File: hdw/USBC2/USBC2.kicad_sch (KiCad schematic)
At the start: 7 parts, among them J1 Conn_01x02, J2 Conn_01x02, J3 Conn_01x02, J4 Conn_01x02, P1 USB_C_2.0

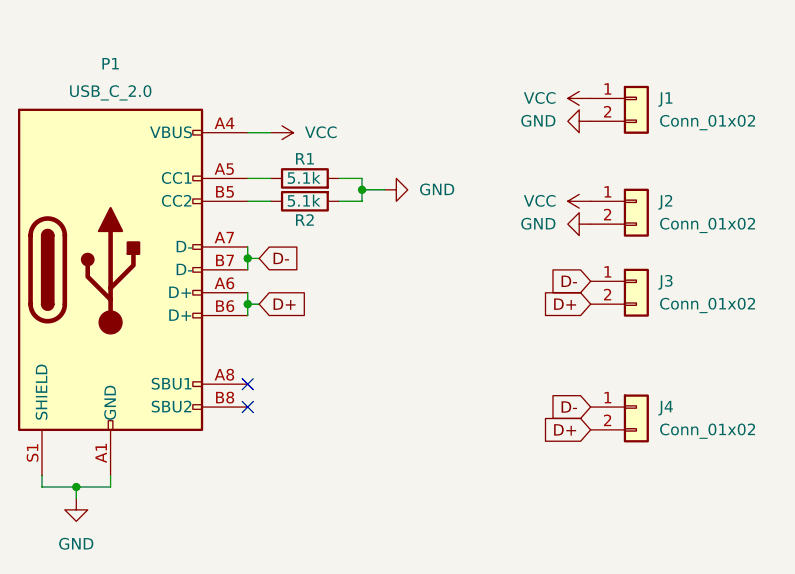
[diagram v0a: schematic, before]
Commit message: Save changes at: 1748195240
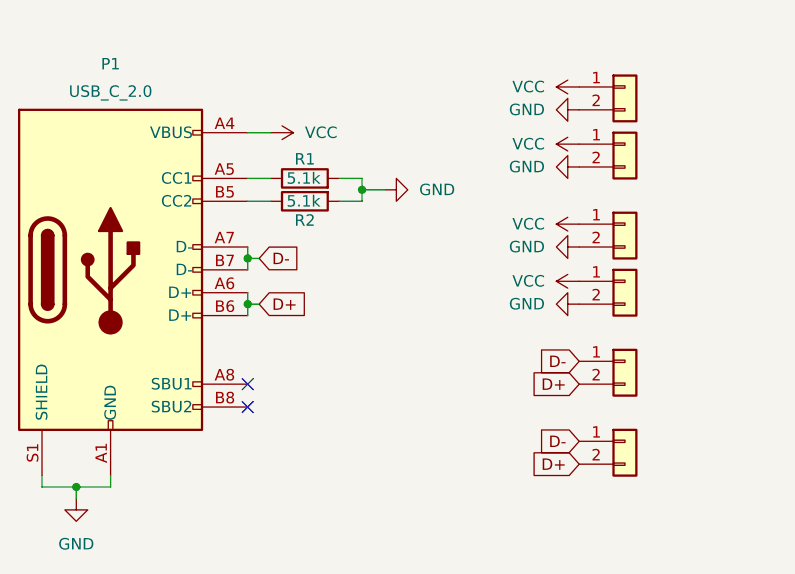
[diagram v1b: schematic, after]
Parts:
- added J5, J6: Conn_01x02, Connector_PinHeader_2.54mm:PinHeader_1x02_P2.54mm_Vertical, symbol Connector_Generic:Conn_01x02
- P1: footprint Connector_USB:USB_C_Receptacle_GCT_USB4105-xx-A_16P_TopMnt_Horizontal -> Connector_USB:USB_C_Receptacle_GCT_USB4085
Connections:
- net GND: now also J5.2 (Pin_2), J6.2 (Pin_2)
- net VCC: now also J5.1 (Pin_1), J6.1 (Pin_1)

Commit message: Save changes at: 1748380927
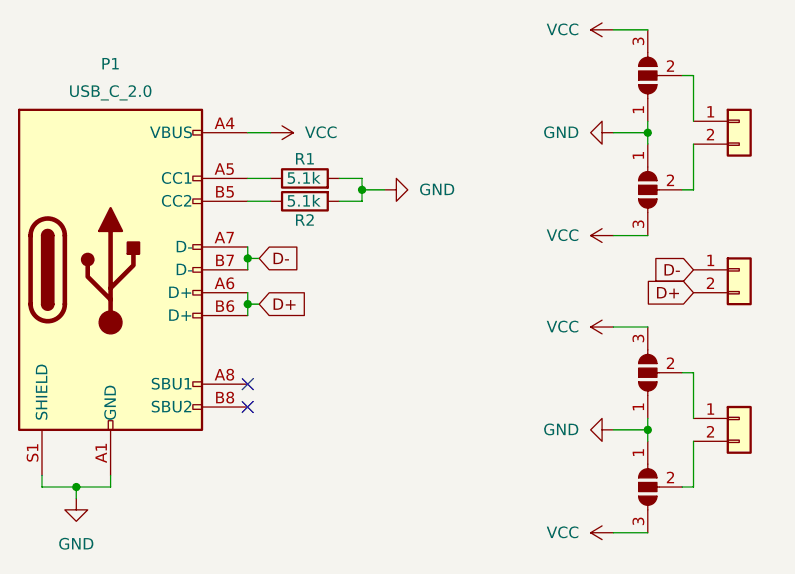
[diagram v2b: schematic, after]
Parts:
- removed J2, J4, J5: Conn_01x02, Connector_PinHeader_2.54mm:PinHeader_1x02_P2.54mm_Vertical, symbol Connector_Generic:Conn_01x02
- added JP5, JP6, JP7, JP8: SolderJumper_3_Open, Jumper:SolderJumper-3_P1.3mm_Open_Pad1.0x1.5mm, symbol Jumper:SolderJumper_3_Open
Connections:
- net GND: now also JP5.1 (A), JP6.1 (A), JP7.1 (A), JP8.1 (A); no longer J1.2 (Pin_2), J6.2 (Pin_2)
- net VCC: now also JP5.3 (B), JP6.3 (B), JP7.3 (B), JP8.3 (B); no longer J1.1 (Pin_1), J6.1 (Pin_1)
- new net: J6.1 (Pin_1), JP7.2 (C)
- new net: J1.1 (Pin_1), JP5.2 (C)
- new net: J1.2 (Pin_2), JP6.2 (C)
- new net: J6.2 (Pin_2), JP8.2 (C)
